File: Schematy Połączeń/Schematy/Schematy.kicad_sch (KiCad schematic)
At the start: 11 parts, among them Q1 2N2219, Q2 2N2219, U1 ESP32-WROOM-32, U2 ESP32-WROOM-32, U3 ESP32-WROOM-32

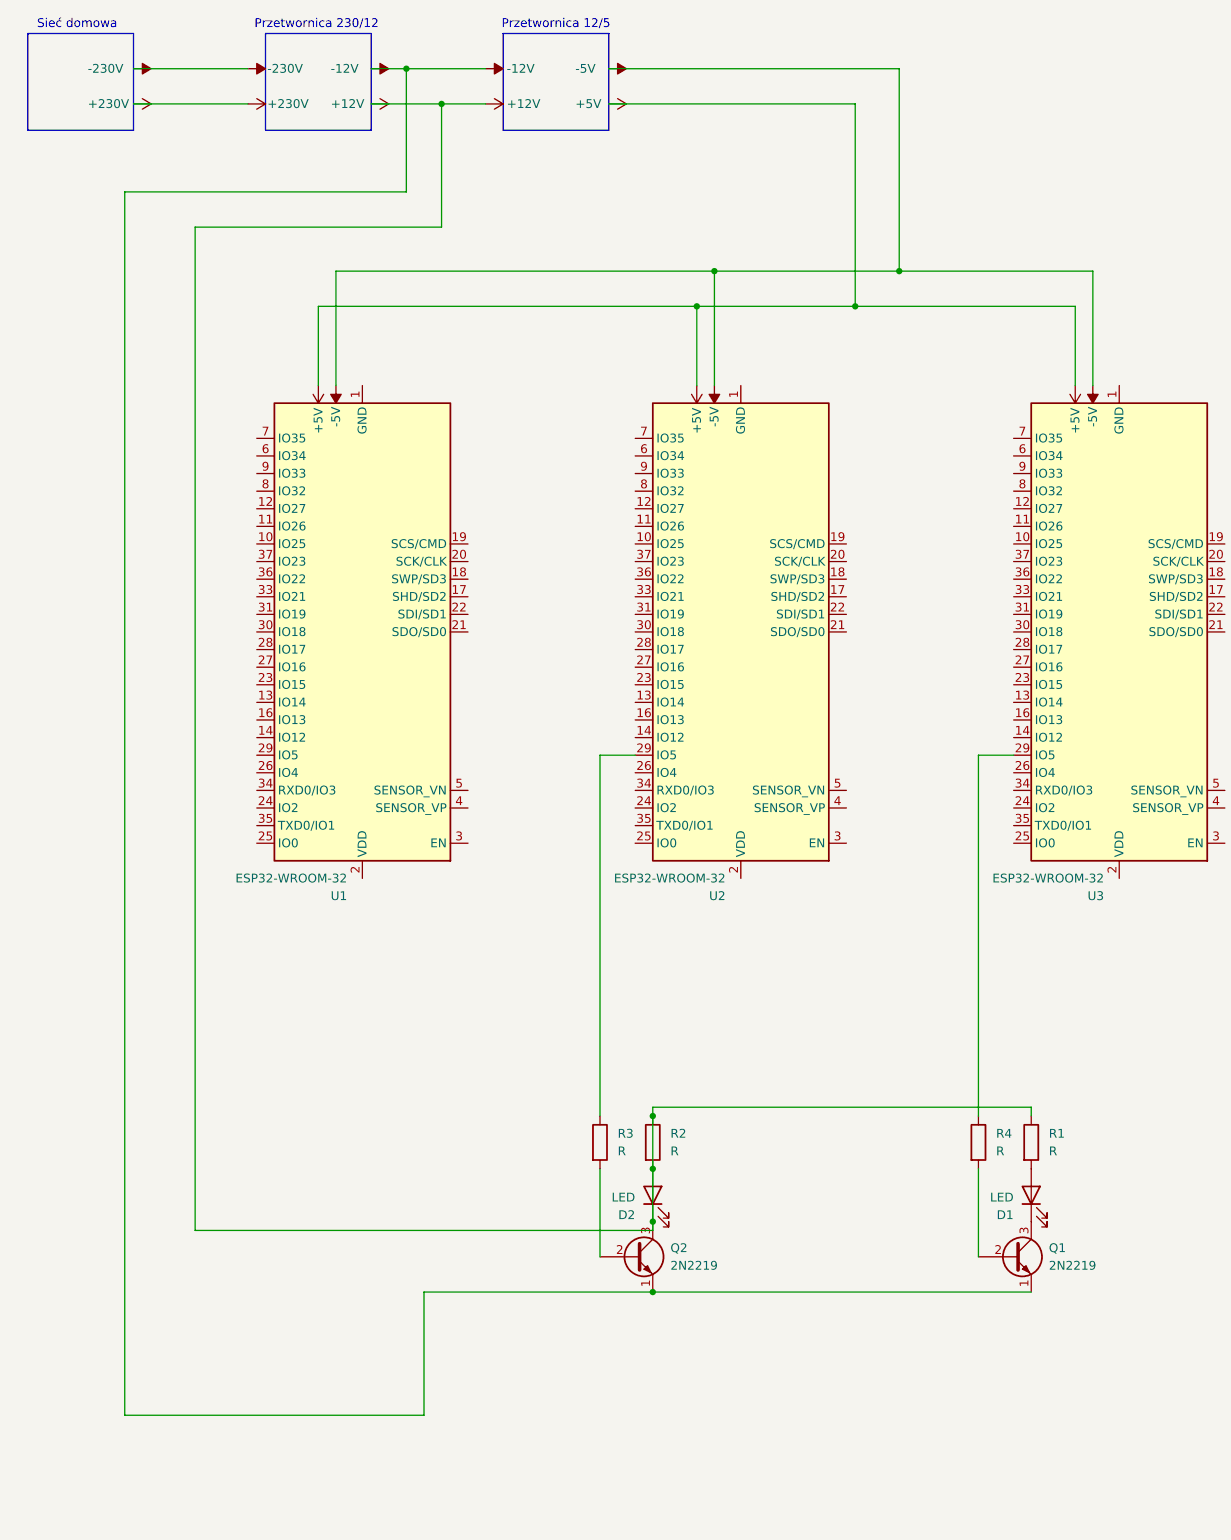
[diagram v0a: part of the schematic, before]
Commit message: Dokument do zaliczenia 7 semestru
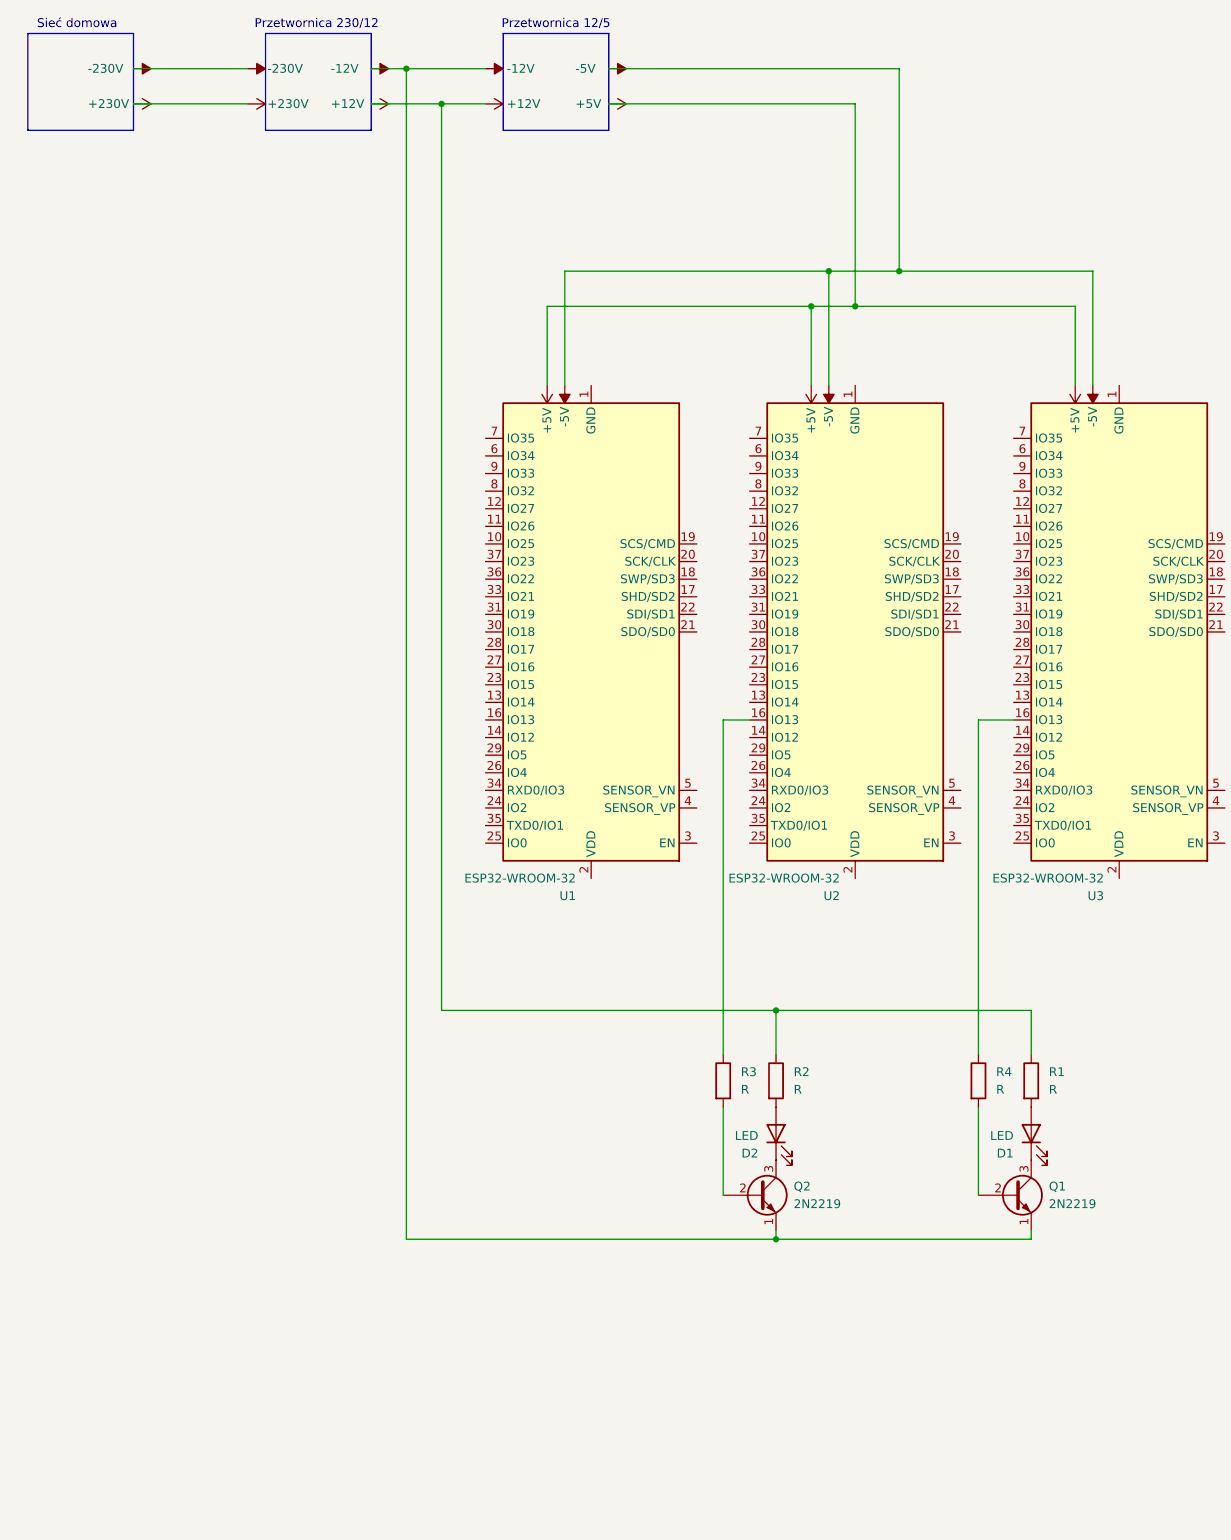
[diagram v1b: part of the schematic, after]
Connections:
- net +12V: no longer D2.1 (K), D2.2 (A), Q2.3 (C), R2.2
- net at R3.1: now also U2.16 (IO13); no longer U2.29 (IO5)
- net at R4.1: now also U3.16 (IO13); no longer U3.29 (IO5)
- new net: D2.1 (K), Q2.3 (C)
- new net: D2.2 (A), R2.2
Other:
- moved on the sheet: D1, D2, Q1, Q2, R1, R2, R3, R4, U1, U2
